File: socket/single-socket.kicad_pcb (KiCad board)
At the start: 2 copper layers, 89 x 89 mm, 180 parts, among them J109 Conn_01x01, J110 Conn_01x01, J111 Conn_01x01, J112 Conn_01x01, J113 Conn_01x01, J114 Conn_01x01, J115 Conn_01x01, J116 Conn_01x01, J117 Conn_01x01, J118 Conn_01x01, J119 Conn_01x01, J120 Conn_01x01, J121 Conn_01x01, J122 Conn_01x01, J123 Conn_01x01, J124 Conn_01x01, J125 Conn_01x01, J126 Conn_01x01, J127 Conn_01x01, J128 Conn_01x01, J129 Conn_01x01, J13 Conn_01x01, J130 Conn_01x01, J131 Conn_01x01, J132 Conn_01x01, J133 Conn_01x01, J134 Conn_01x01, J135 Conn_01x01, J136 Conn_01x01, J137 Conn_01x01, J138 Conn_01x01, J139 Conn_01x01, J14 Conn_01x01, J140 Conn_01x01, J141 Conn_01x01, J142 Conn_01x01, J143 Conn_01x01, J144 Conn_01x01, J145 Conn_01x01, J146 Conn_01x01, J147 Conn_01x01, J148 Conn_01x01, J149 Conn_01x01, J15 Conn_01x01, J150 Conn_01x01, J151 Conn_01x01, J152 Conn_01x01, J153 Conn_01x01, J154 Conn_01x01, J155 Conn_01x01, J156 Conn_01x01, J157 Conn_01x01, J158 Conn_01x01, J159 Conn_01x01, J16 Conn_01x01, J160 Conn_01x01, J161 Conn_01x01, J162 Conn_01x01, J163 Conn_01x01, J164 Conn_01x01, J165 Conn_01x01, J166 Conn_01x01, J167 Conn_01x01, J168 Conn_01x01, J169 Conn_01x01, J17 Conn_01x01, J170 Conn_01x01, J171 Conn_01x01, J172 Conn_01x01, J173 Conn_01x01, J174 Conn_01x01, J175 Conn_01x01, J176 Conn_01x01, J177 Conn_01x01, J178 Conn_01x01, J179 Conn_01x01, J18 Conn_01x01, J180 Conn_01x01, J19 Conn_01x01, J20 Conn_01x01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

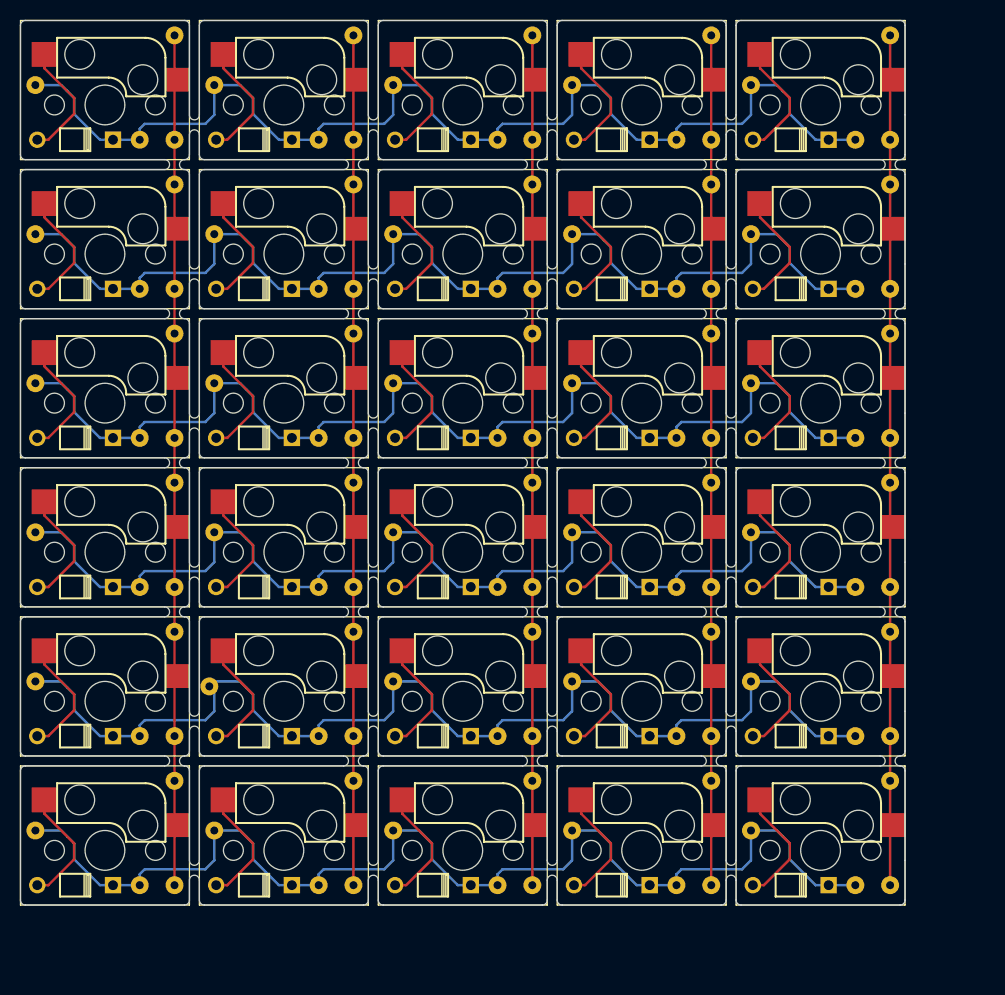
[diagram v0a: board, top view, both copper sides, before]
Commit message: will jlc accept this shit? to be concluded.
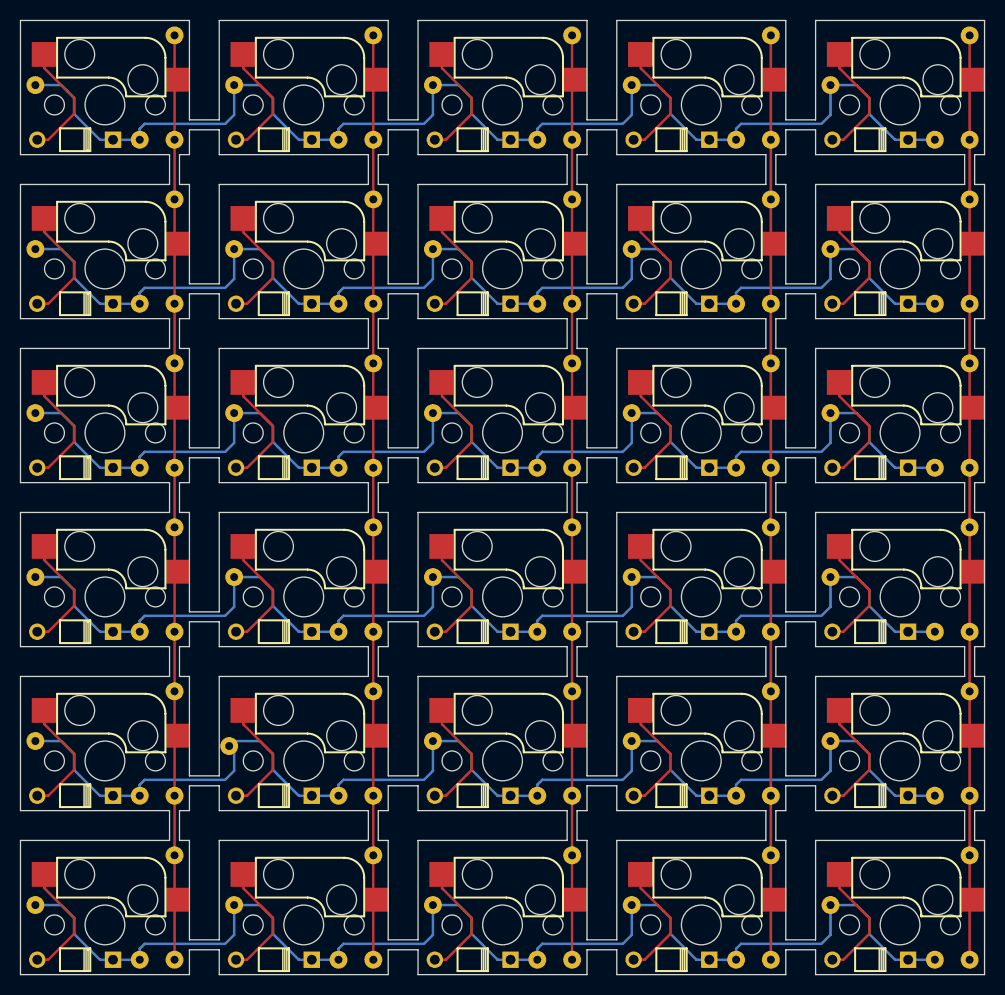
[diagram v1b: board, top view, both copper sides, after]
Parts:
- moved J119 11.0 mm to (127.0, 115.5)
- moved J120 11.0 mm to (127.0, 126.0)
- moved J179 11.0 mm to (113.0, 120.5)
- moved J180 11.0 mm to (123.5, 126.0)
- moved diode30 11.0 mm to (117.0, 126.0)
- moved switch30 11.0 mm to (120.0, 122.5)
- moved J117 10.0 mm to (127.0, 99.0)
- moved J118 10.0 mm to (127.0, 109.5)
- moved J160 10.0 mm to (113.0, 104.0)
- moved J170 10.0 mm to (123.5, 109.5)
- moved diode29 10.0 mm to (117.0, 109.5)
- moved switch29 10.0 mm to (120.0, 106.0)
- moved J177 9.60 mm to (93.0, 120.5)
- moved J178 9.60 mm to (103.5, 126.0)
- moved J95 9.60 mm to (107.0, 115.5)
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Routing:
- net Net-(J129-Pad1): track 117.3 -> 124.9 mm
- net Net-(J171-Pad1): track 117.3 -> 124.9 mm
- net Net-(J125-Pad1): track 117.3 -> 124.9 mm
- net Net-(J127-Pad1): track 117.3 -> 124.9 mm
- net Net-(J123-Pad1): track 117.3 -> 124.9 mm
- net Net-(J121-Pad1): track 117.4 -> 125.0 mm
- net Net-(J85-Pad1): track 87.3 -> 94.8 mm
- net Net-(J61-Pad1): track 87.3 -> 94.8 mm
- net Net-(J13-Pad1): track 87.3 -> 94.8 mm
- net Net-(J109-Pad1): track 87.3 -> 94.8 mm
- net Net-(J37-Pad1): track 87.3 -> 94.8 mm
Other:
- board size 89 x 89 mm -> 97 x 96 mm
